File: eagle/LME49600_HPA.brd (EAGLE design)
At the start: 100 x 80 mm, 41 parts, among them IC1 OPA2134P, IC2 OPA2134P, P1 POLYSWITCH, P2 POLYSWITCH

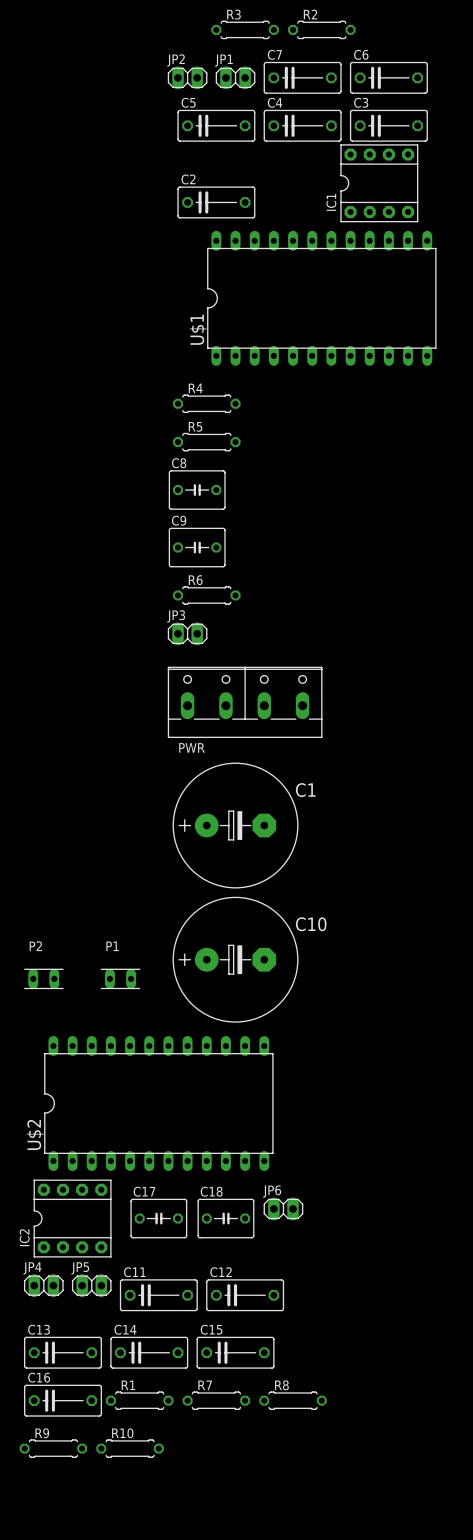
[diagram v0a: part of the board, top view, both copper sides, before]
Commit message: bug fix
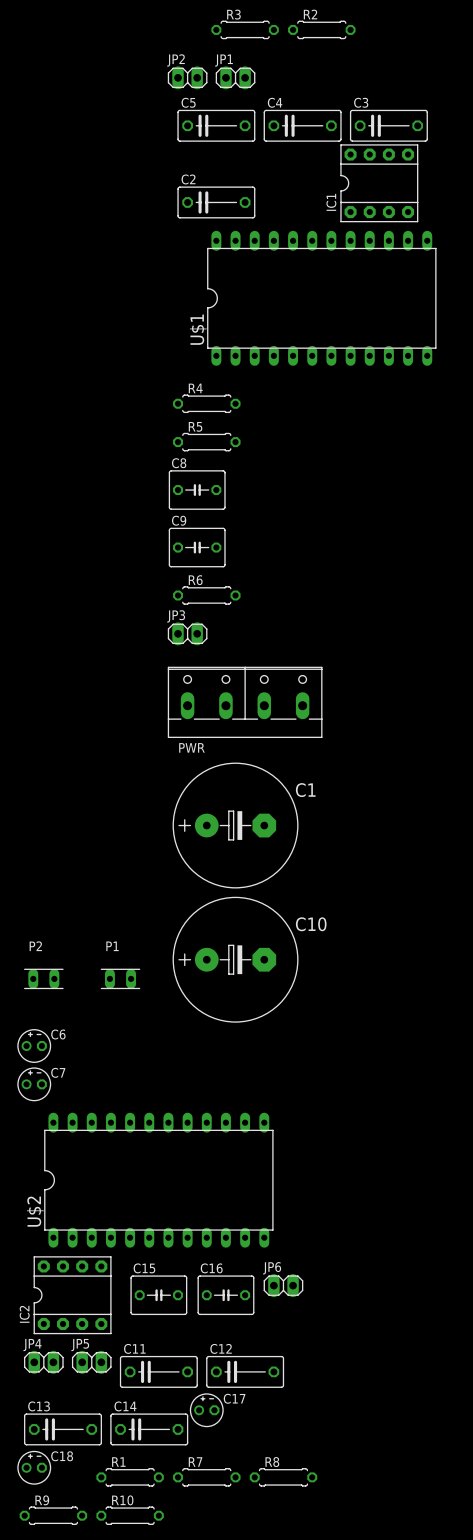
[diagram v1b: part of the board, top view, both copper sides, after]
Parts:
- C15, C16: value 4.7uF -> 1.0uF; device rcl:C075-042X103 -> rcl:C050-050X075
- C17, C18: value 1.0uF -> 4.7uF; device rcl:C050-050X075 -> rcl:E2-4
- C6, C7: device rcl:C075-042X103 -> rcl:E2-4
- moved C7 138.0 mm to (-66.0, -94.0)
- moved C6 136.6 mm to (-66.0, -88.9)
- moved C18 41.7 mm to (-66.0, -144.8)
- moved C17 26.2 mm to (-43.2, -137.2)
- moved C16 25.7 mm to (-40.6, -121.9)
- moved C15 12.7 mm to (-49.5, -121.9)
- moved R1 10.2 mm to (-53.3, -146.1)
- moved R7 10.2 mm to (-43.2, -146.1)
- moved R8 10.2 mm to (-33.0, -146.1)
- moved C11 10.2 mm to (-49.5, -132.1)
- moved C12 10.2 mm to (-38.1, -132.1)
- moved JP6 10.2 mm to (-33.0, -120.7)
- moved U$2 10.2 mm to (-50.8, -106.7)
- moved C13 10.2 mm to (-62.2, -139.7)
- moved C14 10.2 mm to (-50.8, -139.7)
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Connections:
- net N$9 renamed PW-
- net P1 renamed PW+
- removed net N$12 (its old number): C17.2, IC2.7, JP6.1, R10.1
- new net N$9: C16.1, IC2.5, R9.2
- net AGND: now also C17.-, C18.+, C6.-, C7.+; no longer C15.2, C18.2, C6.2, C7.2
- net N$10: now also C15.2, IC2.7, JP6.1, R10.1; no longer C18.1, IC2.6, R9.2
- net N$5: now also C15.1, IC2.6; no longer C17.1, IC2.5
- net N$6: now also IC1.6; no longer IC1.5
- net N$8: now also IC1.5; no longer IC1.6
- net V+: now also C17.+, C6.+; no longer C15.1, C6.1
- net V-: now also C18.-, C7.-; no longer C16.1, C7.1
